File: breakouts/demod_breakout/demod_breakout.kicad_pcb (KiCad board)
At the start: 2 copper layers, 31 parts, among them P1 CONN_02X03, P2 CONN_01X02, U1 CONN_SMA, U2 mounting_box, U3 TCM-63AX+, U4 ADL5380, U5 TCM-63AX+, U6 CONN_SMA, U7 ADM7150

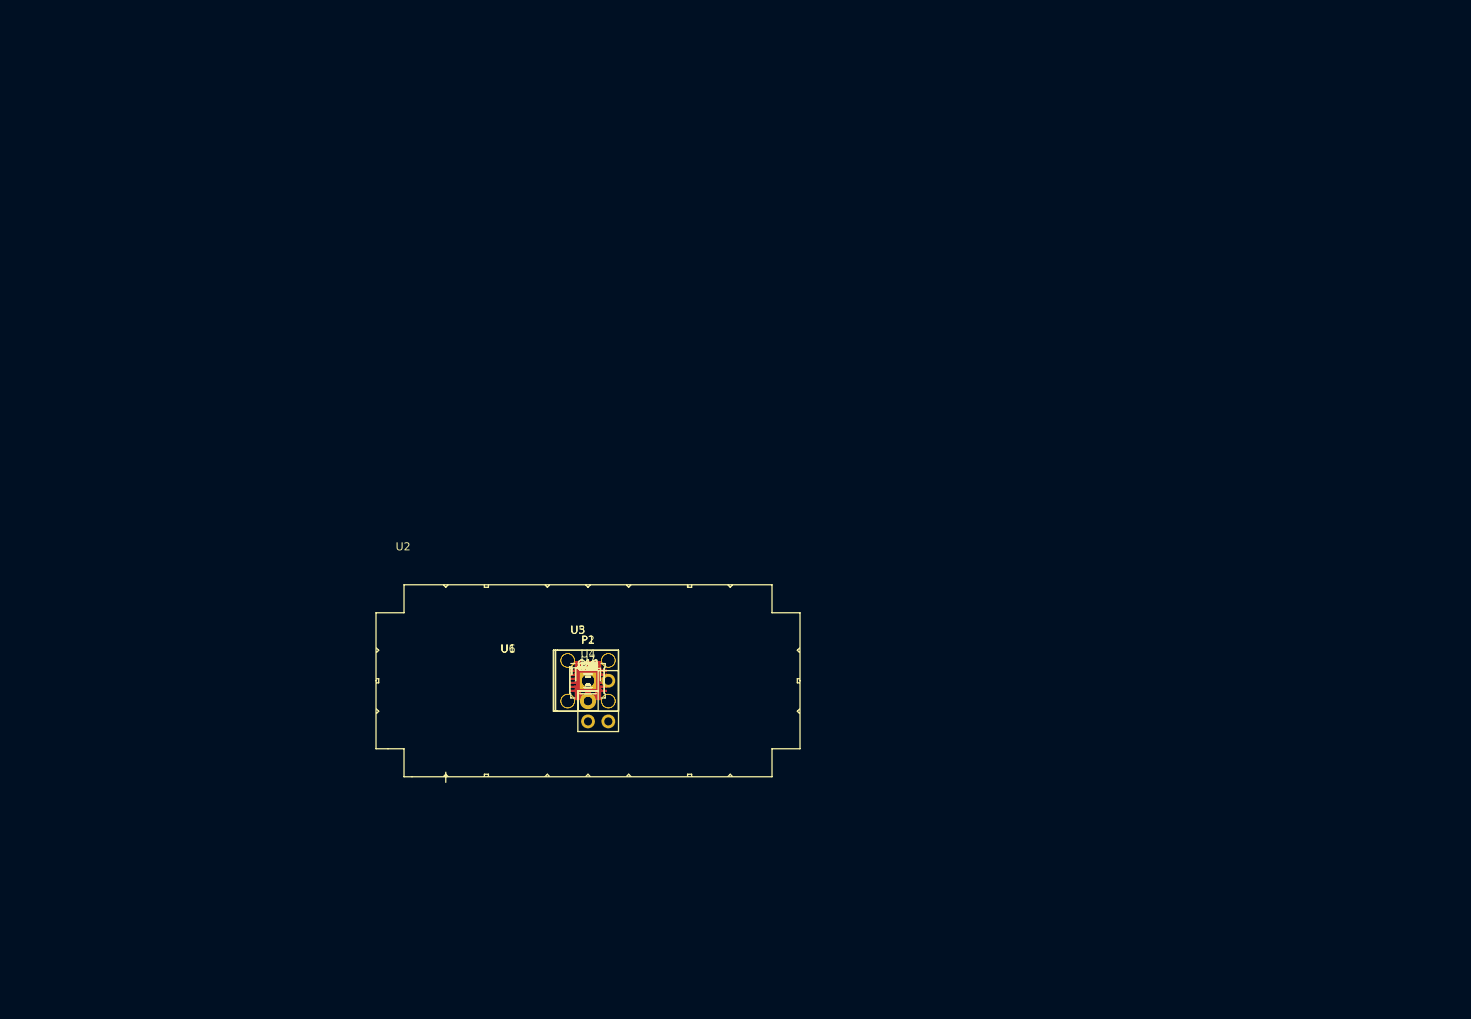
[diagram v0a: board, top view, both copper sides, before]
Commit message: demod component placement
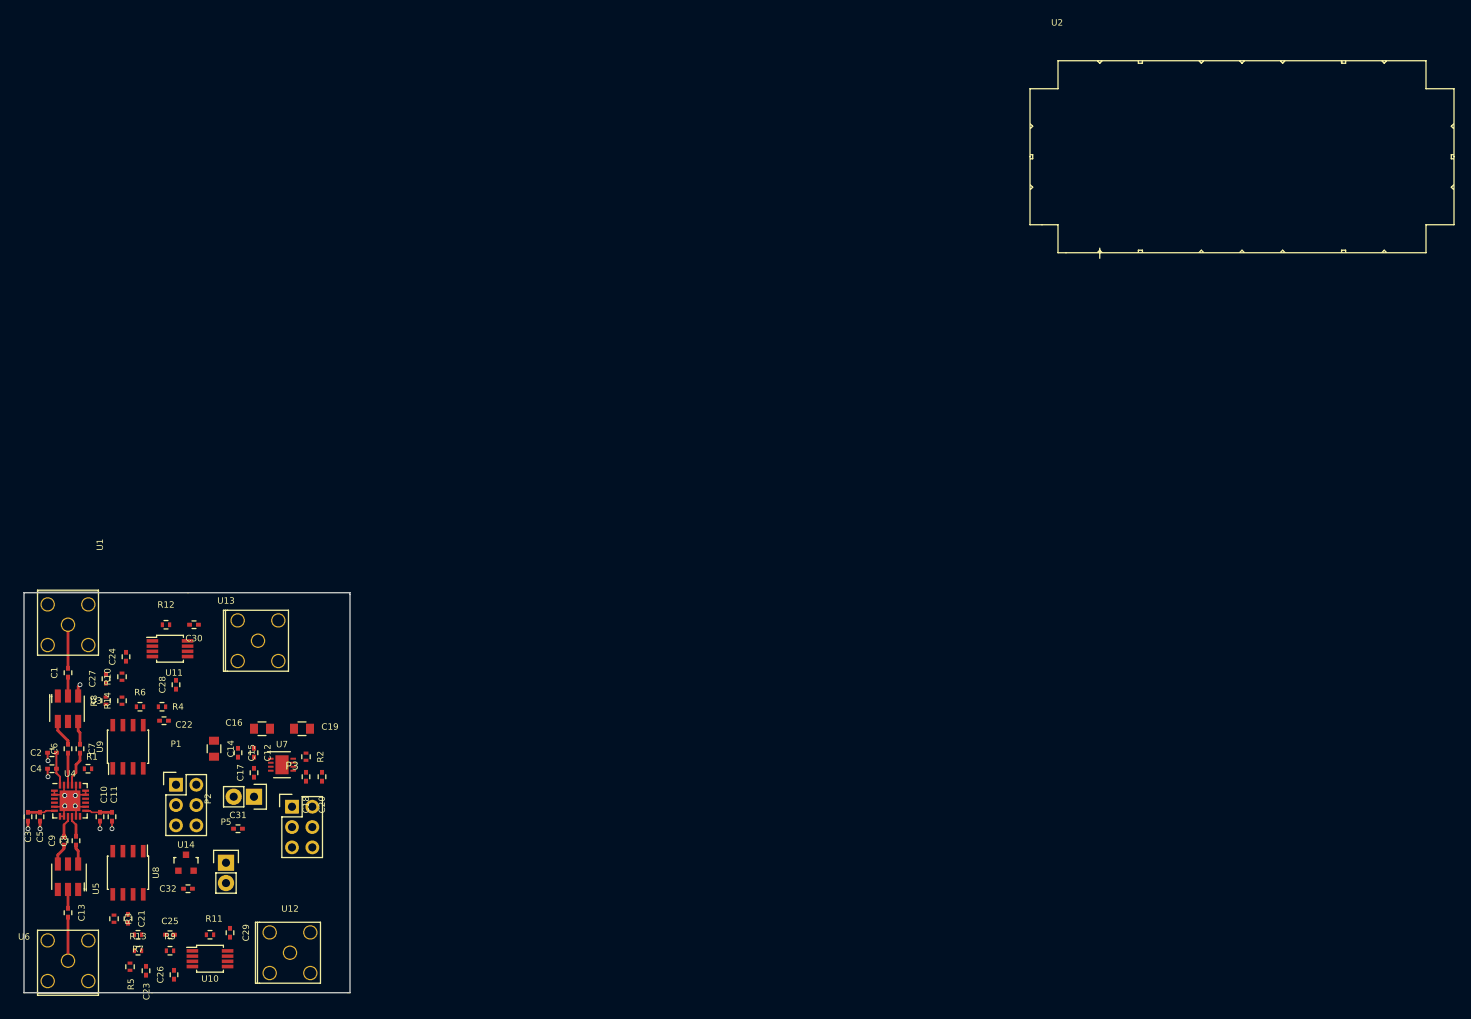
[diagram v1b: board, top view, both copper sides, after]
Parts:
- added C21: 100 nF, Capacitors_SMD:C_0402, F.Cu at (91.0, 134.8)
- added C22: 100 nF, Capacitors_SMD:C_0402, F.Cu at (95.5, 110.0)
- added C23: 100 nF, Capacitors_SMD:C_0402, F.Cu at (93.2, 141.2)
- added C24: 100 nF, Capacitors_SMD:C_0402, F.Cu at (90.8, 102.0)
- added C25: DNP, Capacitors_SMD:C_0402, F.Cu at (96.2, 136.8)
- added C26: 100 nF, Capacitors_SMD:C_0402, F.Cu at (96.8, 141.8)
- added C27: DNP, Capacitors_SMD:C_0402, F.Cu at (88.2, 104.8)
- added C28: 100 nF, Capacitors_SMD:C_0402, F.Cu at (97.0, 105.5)
- added C29: 100 nF, Capacitors_SMD:C_0402, F.Cu at (103.8, 136.5)
- added C30: 100 nF, Capacitors_SMD:C_0402, F.Cu at (99.2, 98.0)
- added C31: 100 nF, Capacitors_SMD:C_0402, F.Cu at (104.8, 123.5)
- added C32: 100 nF, Capacitors_SMD:C_0402, F.Cu at (98.5, 131.0)
- added P3: CONN_02X03, Pin_Headers:Pin_Header_Straight_2x03, F.Cu at (111.5, 120.8)
- added P5: CONN_01X02, Pin_Headers:Pin_Header_Straight_1x02, F.Cu at (103.2, 127.8)
- added R10: 604, Resistors_SMD:R_0402, F.Cu at (90.2, 104.5)
- added R11: 604, Resistors_SMD:R_0402, F.Cu at (101.2, 136.8)
- added R12: 604, Resistors_SMD:R_0402, F.Cu at (95.8, 98.0)
- added R13: 0, Resistors_SMD:R_0402, F.Cu at (92.2, 138.8)
- added R14: 0, Resistors_SMD:R_0402, F.Cu at (90.2, 107.5)
- added R3: 10k, Resistors_SMD:R_0402, F.Cu at (89.2, 134.8)
- added R4: 10k, Resistors_SMD:R_0402, F.Cu at (95.2, 108.2)
- added R5: 10k, Resistors_SMD:R_0402, F.Cu at (91.2, 140.8)
- added R6: 10k, Resistors_SMD:R_0402, F.Cu at (92.5, 108.2)
- added R7: 604, Resistors_SMD:R_0402, F.Cu at (92.2, 136.8)
- added R8: 604, Resistors_SMD:R_0402, F.Cu at (88.2, 107.5)
- added R9: 604, Resistors_SMD:R_0402, F.Cu at (96.2, 138.8)
- added U10: LT1567, Housings_SSOP:MSOP-8_3x3mm_Pitch0.65mm, F.Cu at (101.2, 139.8)
- added U11: LT1567, Housings_SSOP:MSOP-8_3x3mm_Pitch0.65mm, F.Cu at (96.2, 101.0)
- added U12: CONN_SMA, vna_footprints:732512200_SMA, F.Cu at (111.2, 139.0)
- added U13: CONN_SMA, vna_footprints:732512200_SMA, F.Cu at (107.2, 100.0)
- added U14: LD1117S12CTR, TO_SOT_Packages_SMD:SOT-23, F.Cu at (98.2, 127.8)
- added U8: LTC1566-1, Housings_SOIC:SOIC-8_3.9x4.9mm_Pitch1.27mm, F.Cu at (91.0, 129.0)
- added U9: LTC1566-1, Housings_SOIC:SOIC-8_3.9x4.9mm_Pitch1.27mm, F.Cu at (91.0, 113.2)
- C6: footprint Capacitors_SMD:C_0603 -> Capacitors_SMD:C_0402
- moved U2 104.8 mm to (230.2, 39.5)
- moved U6 73.8 mm to (83.5, 140.0), turned to 90 degrees
- moved C3 72.0 mm to (78.5, 122.0), turned to 90 degrees
- moved C13 71.2 mm to (83.5, 134.0), turned to 270 degrees
- moved C5 70.6 mm to (80.0, 122.0), turned to 90 degrees
- moved U5 69.5 mm to (83.5, 129.5), turned to 180 degrees
- moved C9 68.5 mm to (83.0, 125.0), turned to 270 degrees
- moved C4 67.9 mm to (81.5, 116.0)
- moved C2 67.6 mm to (81.5, 114.0)
- moved C8 67.1 mm to (84.5, 125.0), turned to 270 degrees
- moved U4 66.5 mm to (83.8, 120.0)
- moved C6 65.6 mm to (83.5, 113.5), turned to 90 degrees
- moved U1 65.4 mm to (83.5, 98.0), turned to 270 degrees
- moved U3 65.1 mm to (83.5, 108.5)
- moved C1 65.0 mm to (83.5, 104.0), turned to 90 degrees
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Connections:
- P1 pad 1: /BRF_IN -> /ILO_ADL
- P1 pad 2: /BRF_IP -> /IHI_ADL
- P1 pad 5: /BRF_QN -> /QLO_ADL
- P1 pad 6: /BRF_QP -> /QHI_ADL
- U4 pad 21: Net-(C6-Pad1) -> Net-(C7-Pad1)
- U4 pad 22: Net-(C7-Pad1) -> Net-(C6-Pad1)
- U5 pad 2: GND -> Net-(C13-Pad1)
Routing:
- net GND: track 0.00 -> 25.6 mm, vias 0 -> 11
- net +5V: track 0.00 -> 11.0 mm
- net Net-(C1-Pad2): track 0.00 -> 5.45 mm
- net Net-(C13-Pad2): track 0.00 -> 5.45 mm
- net Net-(C7-Pad1): track 0.00 -> 4.41 mm
- net Net-(C6-Pad1): track 0.00 -> 4.00 mm
- net Net-(C6-Pad2): track 0.00 -> 3.39 mm
- net Net-(C7-Pad2): track 0.00 -> 2.96 mm
- net Net-(C9-Pad1): track 0.00 -> 2.71 mm
- net Net-(C8-Pad1): track 0.00 -> 2.71 mm
- net Net-(C9-Pad2): track 0.00 -> 2.68 mm
- net Net-(C8-Pad2): track 0.00 -> 2.47 mm
- net Net-(C1-Pad1): track 0.00 -> 2.36 mm
- net Net-(C13-Pad1): track 0.00 -> 2.36 mm
- added copper zone on In1.Cu, net GND
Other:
- board outline added: 40.8 x 50 mm
- copper layers 2 -> 4
